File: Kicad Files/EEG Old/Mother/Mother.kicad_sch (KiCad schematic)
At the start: 12 parts, among them J1 Conn_01x05_Pin, U1 Teensy4.1

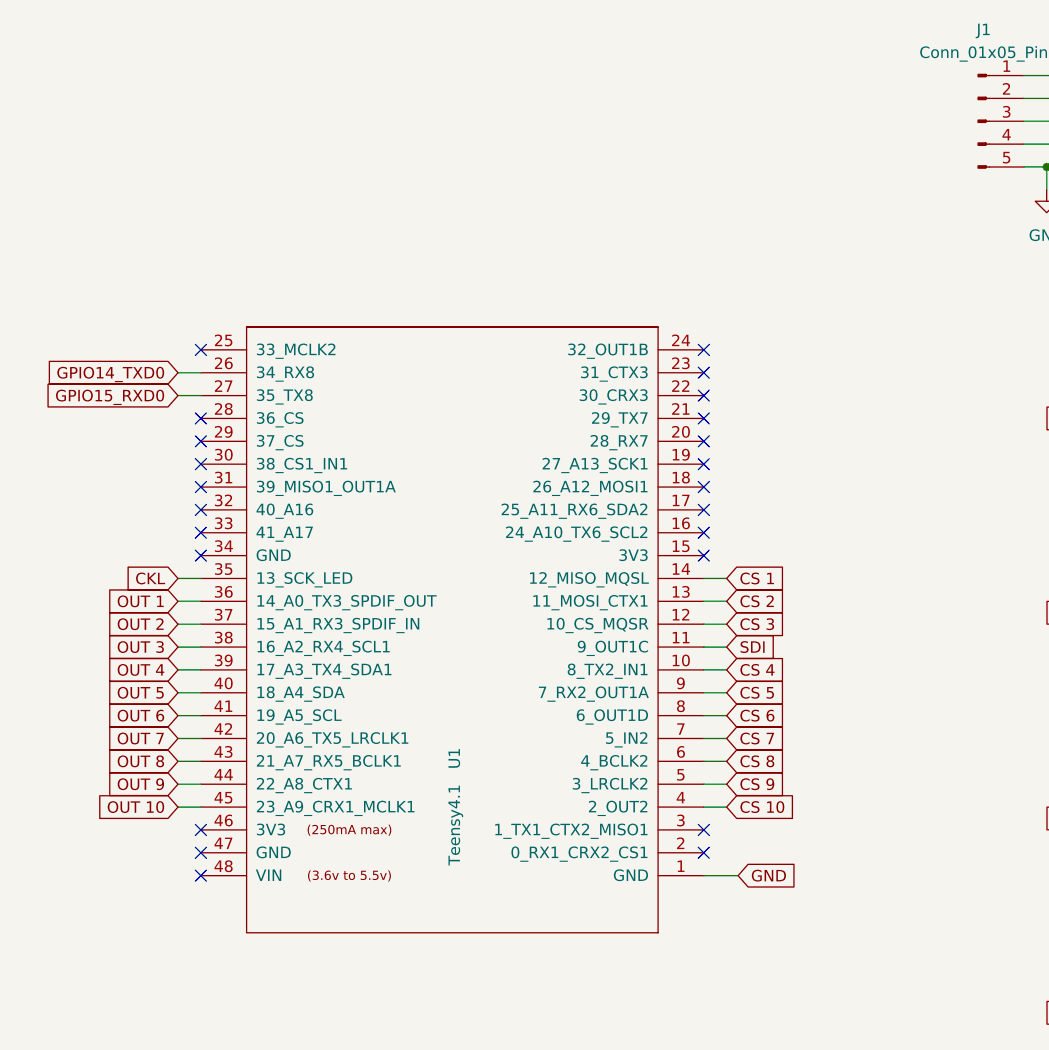
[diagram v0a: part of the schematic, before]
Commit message: EEG Power Updated
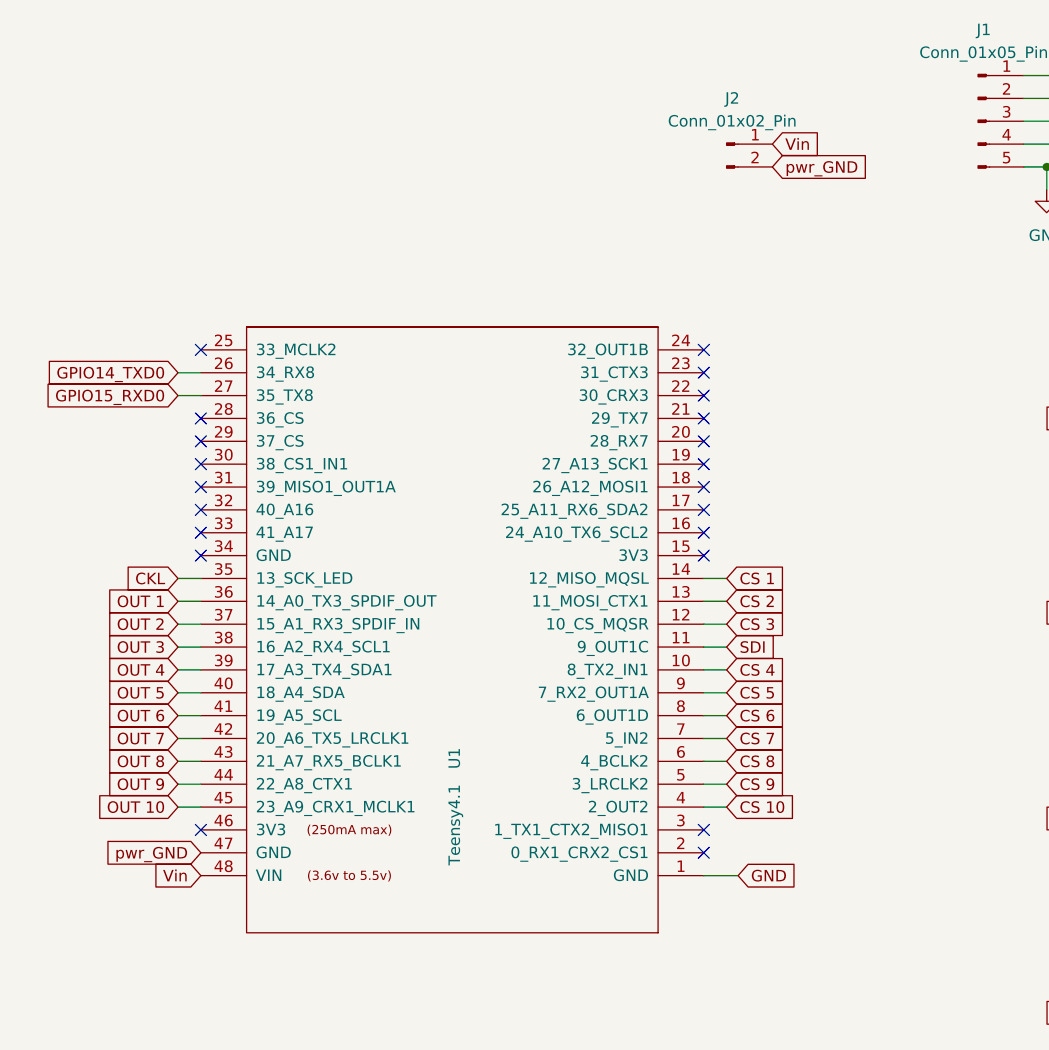
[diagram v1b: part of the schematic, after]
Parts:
- added J2: Conn_01x02_Pin, Connector_PinHeader_1.27mm:PinHeader_1x02_P1.27mm_Vertical, symbol Connector:Conn_01x02_Pin
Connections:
- net pwr_GND: now reaches U1.47 (GND)
- net pwr_GND: now also J2.2 (Pin_2)
- net Vin: now reaches U1.48 (VIN)
- net Vin: now also J2.1 (Pin_1)
- no-connect marks 23 -> 21
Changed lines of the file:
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@@
-	)
-	(no_connect
-		(at 64.77 114.3)
 	)
 	(no_connect
@@
 	(no_connect
 		(at 120.65 111.76)
-	)
-	(no_connect
-		(at 64.77 116.84)
 	)
 	(no_connect
@@
 		)
 	)
+	(global_label "Vin"
+		(shape input)
+		(at 128.27 35.56 0)
+		(fields_autoplaced yes)
+		(effects
+			(font
+				(size 1.27 1.27)
+			)
+			(justify left)
+		)
+		(property "Intersheetrefs" "${INTERSHEET_REFS}"
+			(at 134.0976 35.56 0)
+			(effects
+				(font
+					(size 1.27 1.27)
+				)
+				(justify left)
+				(hide yes)
+			)
+		)
+	)
 	(global_label "SDI"
 		(shape input)
@@
 		)
 	)
+	(global_label "pwr_GND"
+		(shape input)
+		(at 128.27 38.1 0)
+		(fields_autoplaced yes)
+		(effects
+			(font
+				(size 1.27 1.27)
+			)
+			(justify left)
+		)
+		(property "Intersheetrefs" "${INTERSHEET_REFS}"
+			(at 139.359 38.1 0)
+			(effects
+				(font
+					(size 1.27 1.27)
+				)
+				(justify left)
+				(hide yes)
+			)
+		)
+	)
 	(global_label "CS 1"
 		(shape input)
@@
 		)
 	)
+	(global_label "pwr_GND"
+		(shape input)
+		(at 64.77 114.3 180)
+		(fields_autoplaced yes)
+		(effects
+			(font
+				(size 1.27 1.27)
+			)
+			(justify right)
+		)
+		(property "Intersheetrefs" "${INTERSHEET_REFS}"
+			(at 53.681 114.3 0)
+			(effects
+				(font
+					(size 1.27 1.27)
+				)
+				(justify right)
+				(hide yes)
+			)
+		)
+	)
 	(global_label "Vss"
 		(shape input)
@@
 		(property "Intersheetrefs" "${INTERSHEET_REFS}"
 			(at 205.2343 50.8 0)
+			(effects
+				(font
+					(size 1.27 1.27)
+				)
+				(justify right)
+				(hide yes)
+			)
+		)
+	)
+	(global_label "Vin"
+		(shape input)
+		(at 64.77 116.84 180)
+		(fields_autoplaced yes)
+		(effects
+			(font
+				(size 1.27 1.27)
+			)
+			(justify right)
+		)
+		(property "Intersheetrefs" "${INTERSHEET_REFS}"
+			(at 58.9424 116.84 0)
 			(effects
 				(font
@@
 					(unit 1)
 				)
+			)
+		)
+	)
+	(symbol
+		(lib_id "Connector:Conn_01x02_Pin")
+		(at 123.19 35.56 0)
+		(unit 1)
+		(exclude_from_sim no)
+		(in_bom yes)
+		(on_board yes)
+		(dnp no)
+		(fields_autoplaced yes)
+		(property "Reference" "J2"
+			(at 123.825 30.48 0)
+			(effects
+				(font
+					(size 1.27 1.27)
+				)
+			)
+		)
+		(property "Value" "Conn_01x02_Pin"
+			(at 123.825 33.02 0)
+			(effects
+				(font
+					(size 1.27 1.27)
+				)
+			)
+		)
+		(property "Footprint" "Connector_PinHeader_1.27mm:PinHeader_1x02_P1.27mm_Vertical"
+			(at 123.19 35.56 0)
+			(effects
+				(font
+					(size 1.27 1.27)
+				)
+				(hide yes)
+			)
+		)
+		(property "Datasheet" "~"
+			(at 123.19 35.56 0)
+			(effects
+				(font
+					(size 1.27 1.27)
+				)
+				(hide yes)
+			)
+		)
+		(property "Description" "Generic connector, single row, 01x02, script generated"
+			(at 123.19 35.56 0)
+			(effects
+				(font
+					(size 1.27 1.27)
+				)
+				(hide yes)
+			)
+		)
+		(pin "2"
+		)
+		(pin "1"
+		)
+		(instances
+			(project ""
+				(path "/cea3ca6f-b7d1-43d8-9867-cd2ab3cb5e64"
+					(reference "J2")
+					(unit 1)
+				)
